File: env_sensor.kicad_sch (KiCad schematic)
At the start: 47 parts, among them J1 E Paper, J10 PWMOUT, J3 Barrel_Jack, J4 LED_OUTPUT, J5 RegSense, J6 I2c, J7 USB_C_Receptacle_USB2.0_16P, J8 v5_v3, J9 DEBUG, Q1 NMOS, Q2 NMOS, Q3 NMOS, SW1 EN, SW2 BOOT, U1 MH-Z19B, U3 ESP32-S3-WROOM-1, U4 TXB0104PW, U5 BME280, U6 TPS2065CDBV, U7 AP7361C-33E, Y1 Crystal

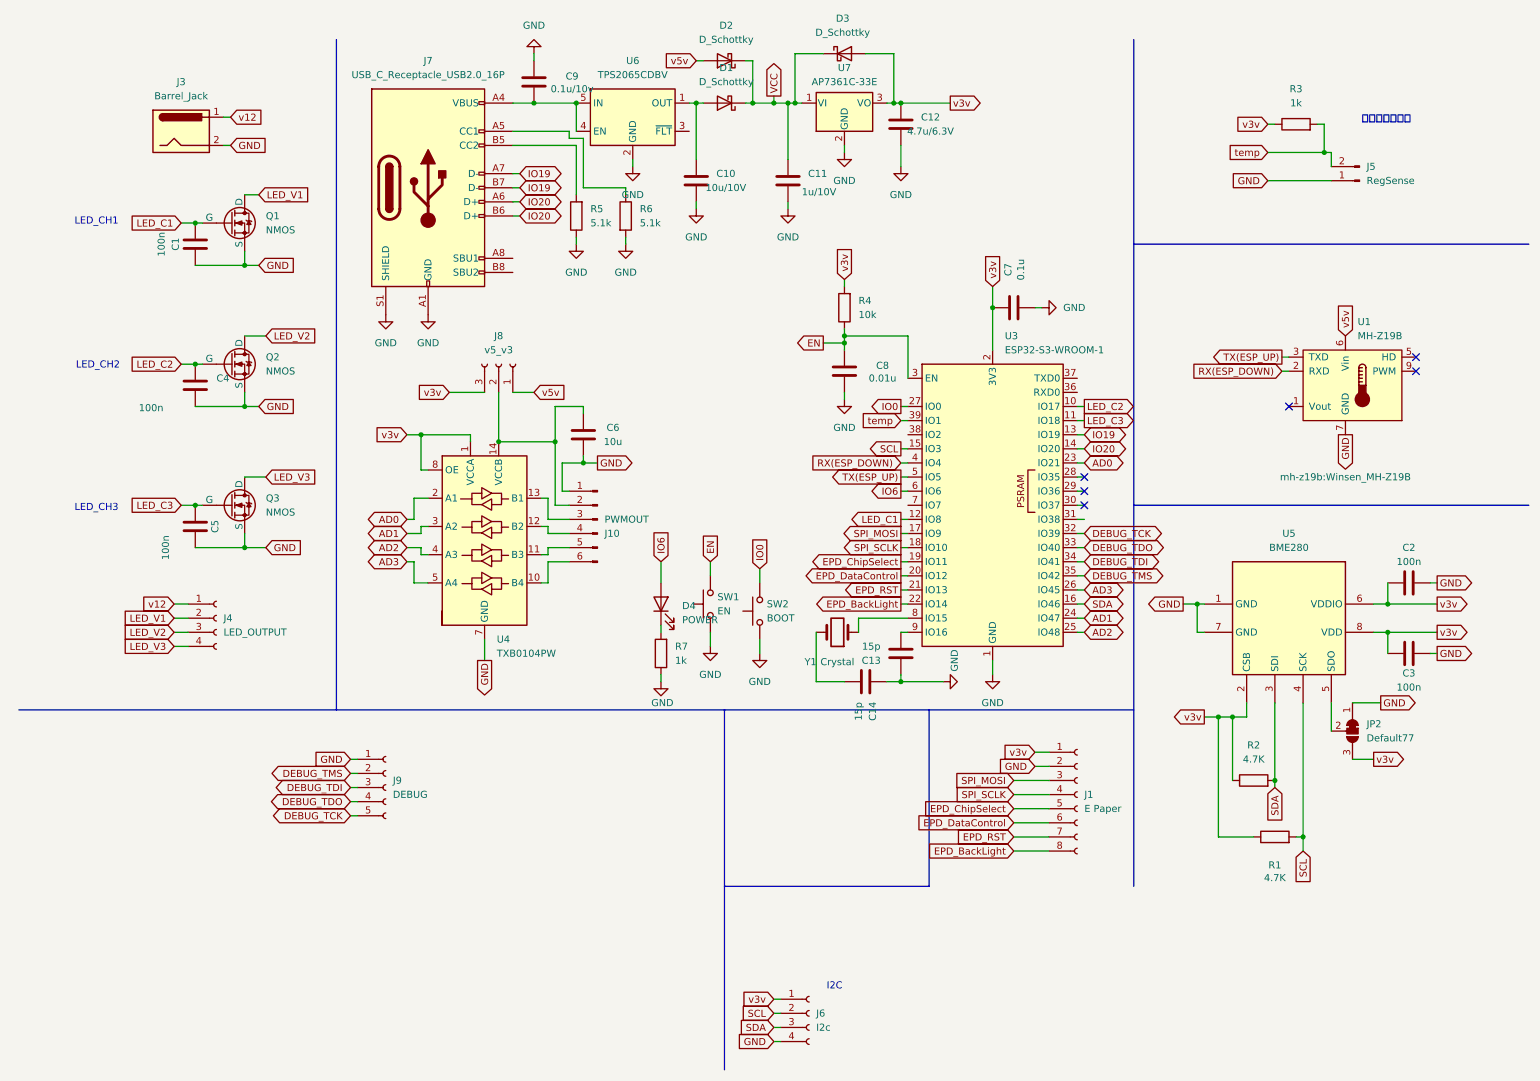
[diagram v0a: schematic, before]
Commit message: update
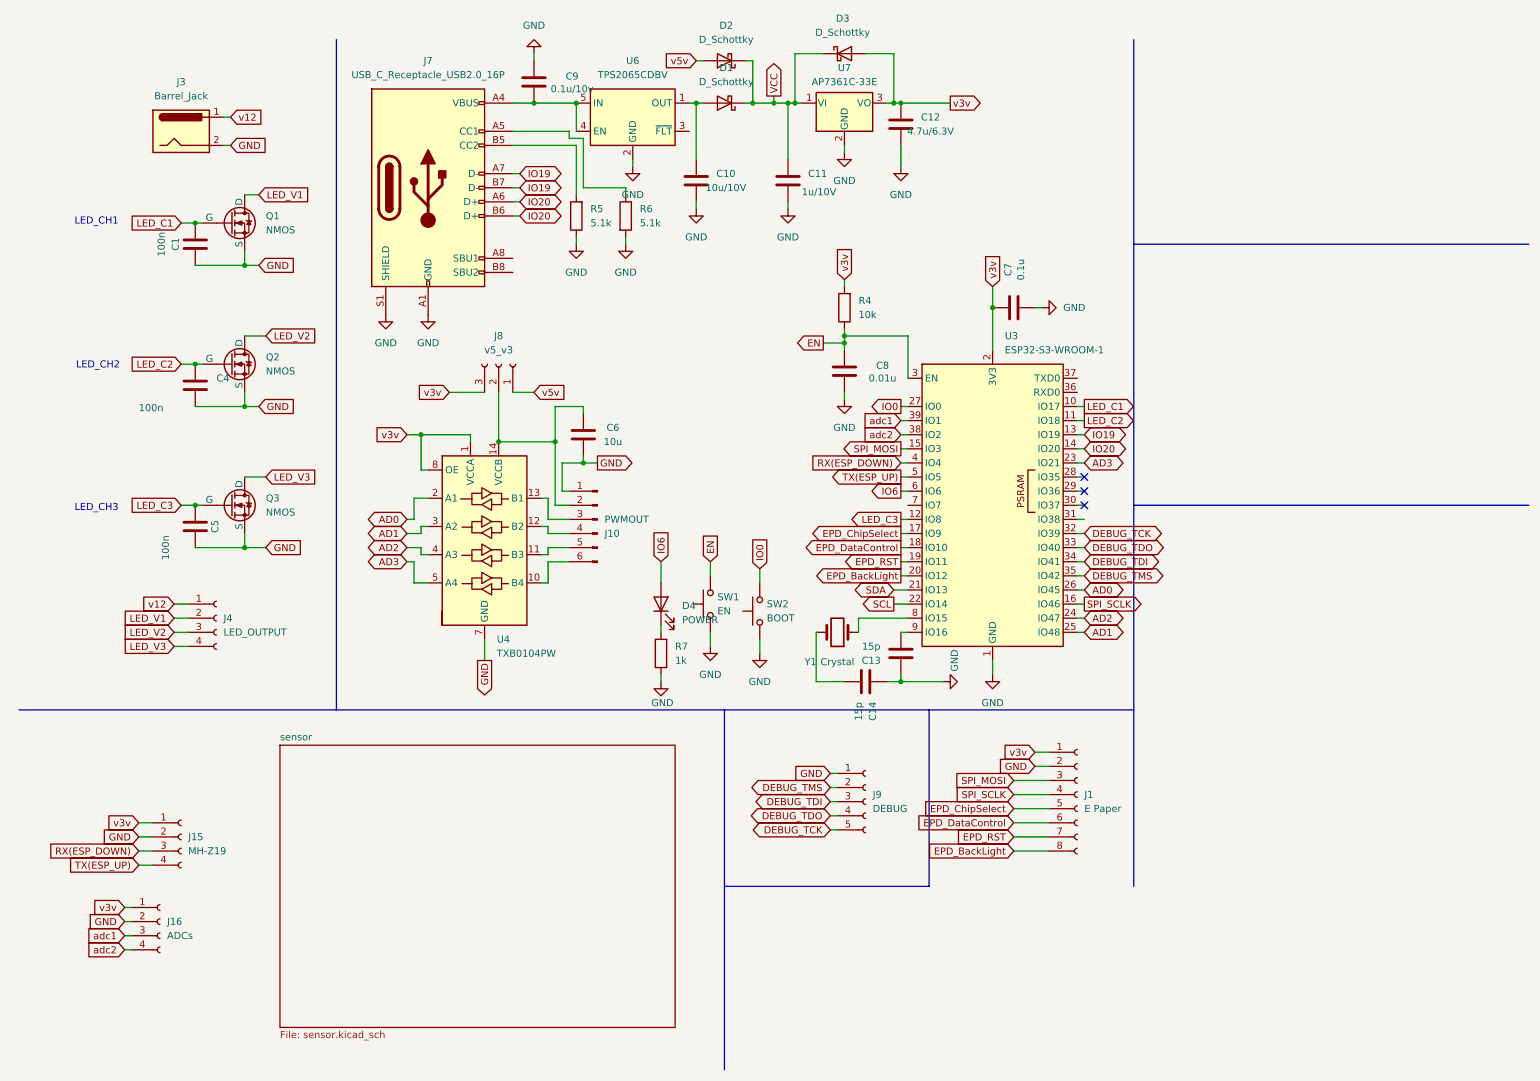
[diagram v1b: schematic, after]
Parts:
- removed C2, C3: 100n, Capacitor_SMD:C_0603_1608Metric, symbol Device:C
- removed J5: RegSense, Connector_PinSocket_2.54mm:PinSocket_1x02_P2.54mm_Vertical, symbol Connector:Conn_01x02_Pin
- removed J6: I2c, Connector_PinSocket_2.54mm:PinSocket_1x04_P2.54mm_Vertical, symbol Connector:Conn_01x04_Socket
- removed JP2: Default77, Jumper:SolderJumper-3_P1.3mm_Bridged12_RoundedPad1.0x1.5mm, symbol Jumper:SolderJumper_3_Bridged12
- removed R1, R2: 4.7K, Resistor_SMD:R_0603_1608Metric, symbol Device:R
- removed R3: 1k, Resistor_SMD:R_0603_1608Metric, symbol Device:R
- removed U1: MH-Z19B, mh-z19b:Winsen_MH-Z19B, symbol mh_z19b:MH-Z19B
- removed U5: BME280, Package_LGA:Bosch_LGA-8_2.5x2.5mm_P0.65mm_ClockwisePinNumbering, symbol Sensor:BME280
- added J15: MH-Z19, Connector_PinSocket_2.54mm:PinSocket_1x04_P2.54mm_Vertical, symbol Connector:Conn_01x04_Socket
- added J16: ADCs, Connector_PinSocket_2.54mm:PinSocket_1x04_P2.54mm_Vertical, symbol Connector:Conn_01x04_Socket
- Q1, Q2: footprint env-sensor:SOT-23 -> env-sensor:TO-252
- Q3: footprint env-sensor:SOT-23 -> env-sensor:TO-252; LCSC C916396 -> C557932
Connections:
- net AD0: now also U3.26 (IO45); no longer U3.23 (IO21)
- net AD1: now also U3.25 (IO48); no longer U3.24 (IO47)
- net AD2: now also U3.24 (IO47); no longer U3.25 (IO48)
- net AD3: now also U3.23 (IO21); no longer U3.26 (IO45)
- net EPD_BackLight: now also U3.20 (IO12); no longer U3.22 (IO14)
- net EPD_ChipSelect: now also U3.17 (IO9); no longer U3.19 (IO11)
- net EPD_DataControl: now also U3.18 (IO10); no longer U3.20 (IO12)
- net EPD_RST: now also U3.19 (IO11); no longer U3.21 (IO13)
- net GND: now also J15.2 (Pin_2), J16.2 (Pin_2)
- net LED_C1: now also U3.10 (IO17); no longer U3.12 (IO8)
- net LED_C2: now also U3.11 (IO18); no longer U3.10 (IO17)
- net LED_C3: now also U3.12 (IO8); no longer U3.11 (IO18)
- net RX(ESP_DOWN): now also J15.3 (Pin_3)
- net SCL: now also U3.22 (IO14); no longer U3.15 (IO3)
- net SDA: now also U3.21 (IO13); no longer U3.16 (IO46)
- net SPI_MOSI: now also U3.15 (IO3); no longer U3.17 (IO9)
- net SPI_SCLK: now also U3.16 (IO46); no longer U3.18 (IO10)
- net TX(ESP_UP): now also J15.4 (Pin_4)
- net v3v: now also J15.1 (Pin_1), J16.1 (Pin_1)
- net adc2: now reaches U3.38 (IO2)
- net adc2: now also J16.4 (Pin_4)
- net temp renamed adc1
- net adc1: now also J16.3 (Pin_3)
- no-connect marks 6 -> 3
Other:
- added sheet sensor (sensor.kicad_sch)
- note removed: "I2C"
- note removed: "サーミスタ回路"
- moved on the sheet: J9

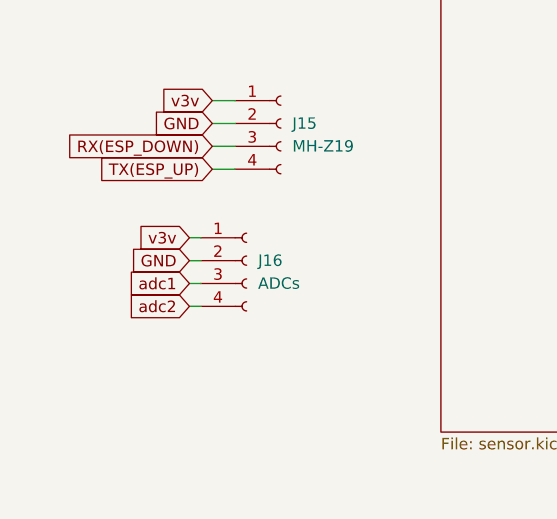
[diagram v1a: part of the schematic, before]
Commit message: fin
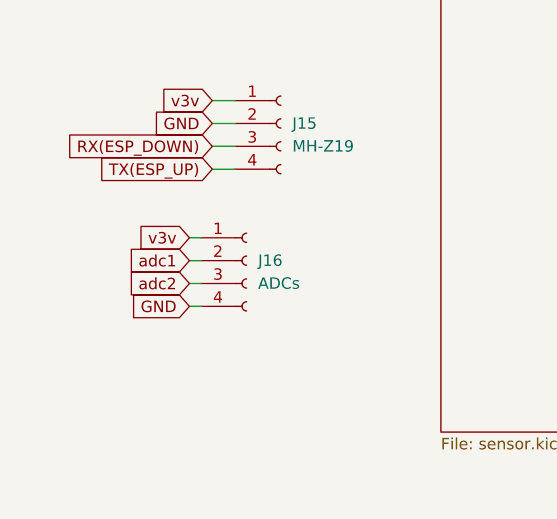
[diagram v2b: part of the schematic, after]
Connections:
- net GND: now also J16.4 (Pin_4); no longer J16.2 (Pin_2)
- net adc1: now also J16.2 (Pin_2); no longer J16.3 (Pin_3)
- net adc2: now also J16.3 (Pin_3); no longer J16.4 (Pin_4)
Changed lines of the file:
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@@
+		)
+	)
+	(global_label "adc2"
+		(shape input)
+		(at 31.75 173.99 180)
+		(fields_autoplaced yes)
+		(effects
+			(font
+				(size 1.27 1.27)
+			)
+			(justify right)
+		)
+		(property "Intersheetrefs" "${INTERSHEET_REFS}"
+			(at 24.1687 173.99 0)
+			(effects
+				(font
+					(size 1.27 1.27)
+				)
+				(justify right)
+				(hide yes)
+			)
 		)
 	)
@@
 		)
 	)
-	(global_label "adc1"
-		(shape input)
-		(at 31.75 173.99 180)
-		(fields_autoplaced yes)
-		(effects
-			(font
-				(size 1.27 1.27)
-			)
-			(justify right)
-		)
-		(property "Intersheetrefs" "${INTERSHEET_REFS}"
-			(at 24.1687 173.99 0)
-			(effects
-				(font
-					(size 1.27 1.27)
-				)
-				(justify right)
-				(hide yes)
-			)
-		)
-	)
 	(global_label "GND"
 		(shape input)
@@
 		)
 	)
-	(global_label "adc2"
-		(shape input)
-		(at 31.75 176.53 180)
-		(fields_autoplaced yes)
-		(effects
-			(font
-				(size 1.27 1.27)
-			)
-			(justify right)
-		)
-		(property "Intersheetrefs" "${INTERSHEET_REFS}"
-			(at 24.1687 176.53 0)
-			(effects
-				(font
-					(size 1.27 1.27)
-				)
-				(justify right)
-				(hide yes)
-			)
-		)
-	)
 	(global_label "LED_C1"
 		(shape input)
@@
 		)
 	)
+	(global_label "v5v"
+		(shape input)
+		(at 134.62 16.51 180)
+		(fields_autoplaced yes)
+		(effects
+			(font
+				(size 1.27 1.27)
+			)
+			(justify right)
+		)
+		(property "Intersheetrefs" "${INTERSHEET_REFS}"
+			(at 128.4901 16.51 0)
+			(effects
+				(font
+					(size 1.27 1.27)
+				)
+				(justify right)
+				(hide yes)
+			)
+		)
+	)
+	(global_label "adc1"
+		(shape input)
+		(at 31.75 171.45 180)
+		(fields_autoplaced yes)
+		(effects
+			(font
+				(size 1.27 1.27)
+			)
+			(justify right)
+		)
+		(property "Intersheetrefs" "${INTERSHEET_REFS}"
+			(at 24.1687 171.45 0)
+			(effects
+				(font
+					(size 1.27 1.27)
+				)
+				(justify right)
+				(hide yes)
+			)
+		)
+	)
+	(global_label "EPD_ChipSelect"
+		(shape input)
+		(at 191.77 151.13 180)
+		(fields_autoplaced yes)
+		(effects
+			(font
+				(size 1.27 1.27)
+			)
+			(justify right)
+		)
+		(property "Intersheetrefs" "${INTERSHEET_REFS}"
+			(at 174.0892 151.13 0)
+			(effects
+				(font
+					(size 1.27 1.27)
+				)
+				(justify right)
+				(hide yes)
+			)
+		)
+	)
 	(global_label "GND"
 		(shape input)
-		(at 31.75 171.45 180)
-		(fields_autoplaced yes)
-		(effects
-			(font
-				(size 1.27 1.27)
-			)
-			(justify right)
-		)
-		(property "Intersheetrefs" "${INTERSHEET_REFS}"
-			(at 24.8943 171.45 0)
-			(effects
-				(font
-					(size 1.27 1.27)
-				)
-				(justify right)
-				(hide yes)
-			)
-		)
-	)
-	(global_label "v5v"
-		(shape input)
-		(at 134.62 16.51 180)
-		(fields_autoplaced yes)
-		(effects
-			(font
-				(size 1.27 1.27)
-			)
-			(justify right)
-		)
-		(property "Intersheetrefs" "${INTERSHEET_REFS}"
-			(at 128.4901 16.51 0)
-			(effects
-				(font
-					(size 1.27 1.27)
-				)
-				(justify right)
-				(hide yes)
-			)
-		)
-	)
-	(global_label "EPD_ChipSelect"
-		(shape input)
-		(at 191.77 151.13 180)
-		(fields_autoplaced yes)
-		(effects
-			(font
-				(size 1.27 1.27)
-			)
-			(justify right)
-		)
-		(property "Intersheetrefs" "${INTERSHEET_REFS}"
-			(at 174.0892 151.13 0)
-			(effects
-				(font
+		(at 31.75 176.53 180)
+		(fields_autoplaced yes)
+		(effects
+			(font
+				(size 1.27 1.27)
+			)
+			(justify right)
+		)
+		(property "Intersheetrefs" "${INTERSHEET_REFS}"
+			(at 24.8943 176.53 0)
+			(effects
+				(font

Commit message: update lib for switch and fix DRCs
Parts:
- SW1, SW2: footprint (none) -> paripalpp_button:TVAF06-A020B-R
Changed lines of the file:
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@@
 			)
 		)
-		(property "Footprint" ""
+		(property "Footprint" "paripalpp_button:TVAF06-A020B-R"
 			(at 140.97 115.57 0)
 			(effects
@@
 			)
 		)
-		(property "Footprint" ""
+		(property "Footprint" "paripalpp_button:TVAF06-A020B-R"
 			(at 132.08 114.3 0)
 			(effects

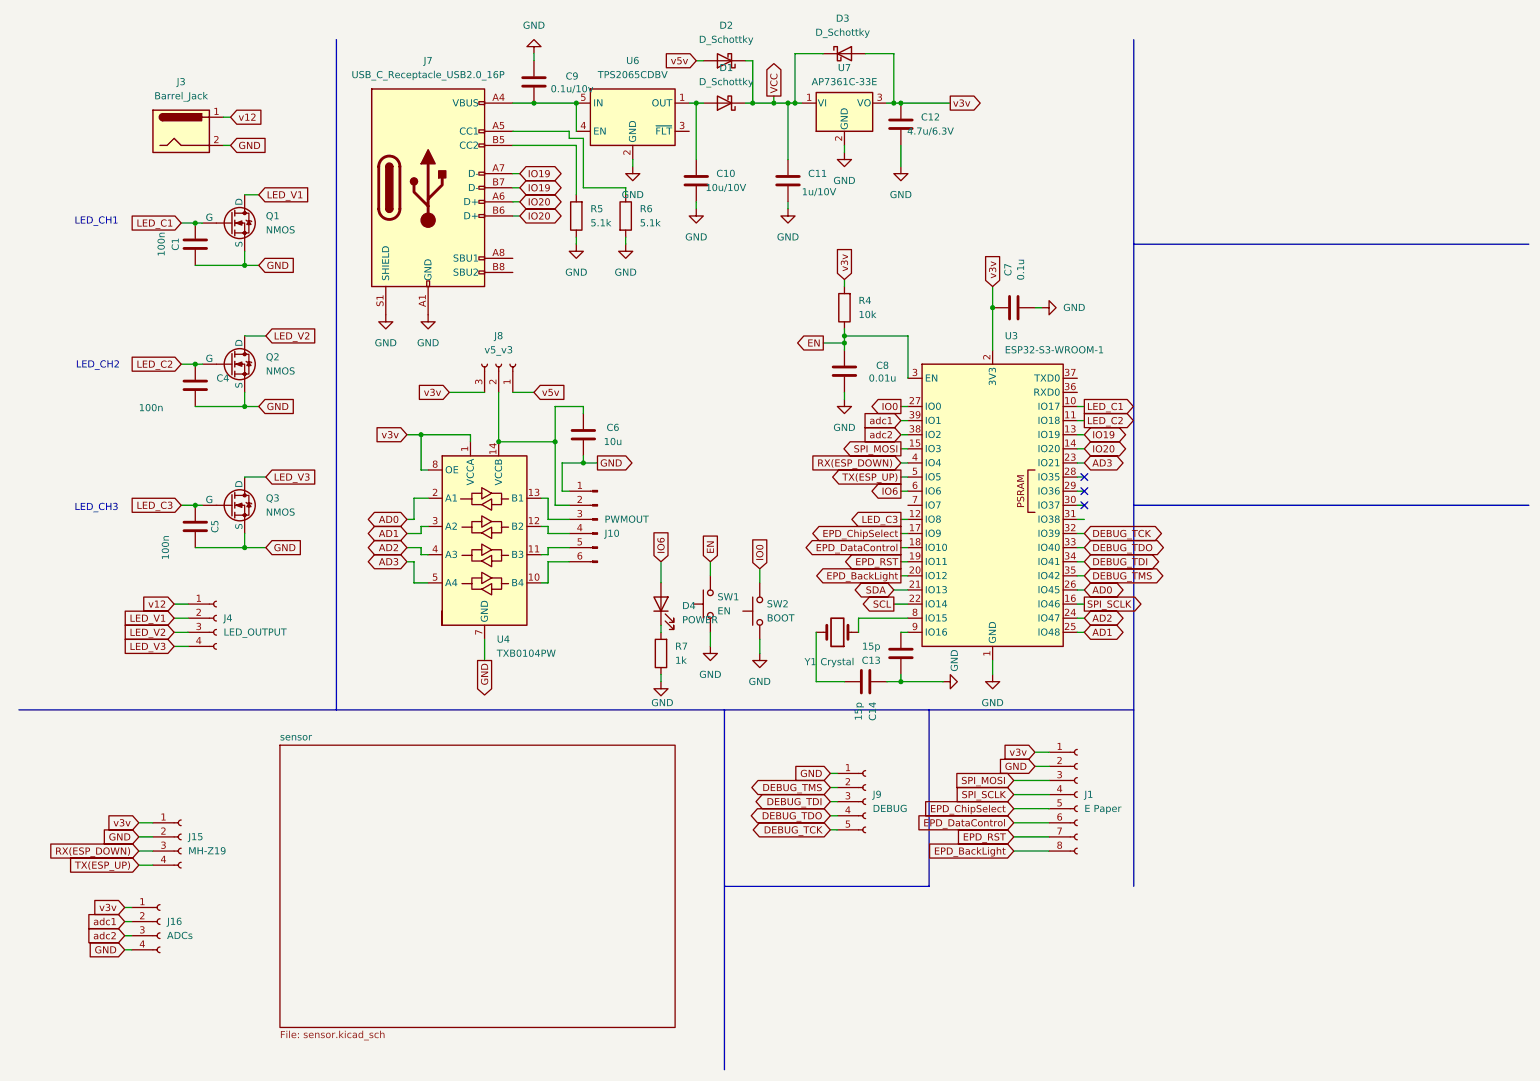
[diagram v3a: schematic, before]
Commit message: update
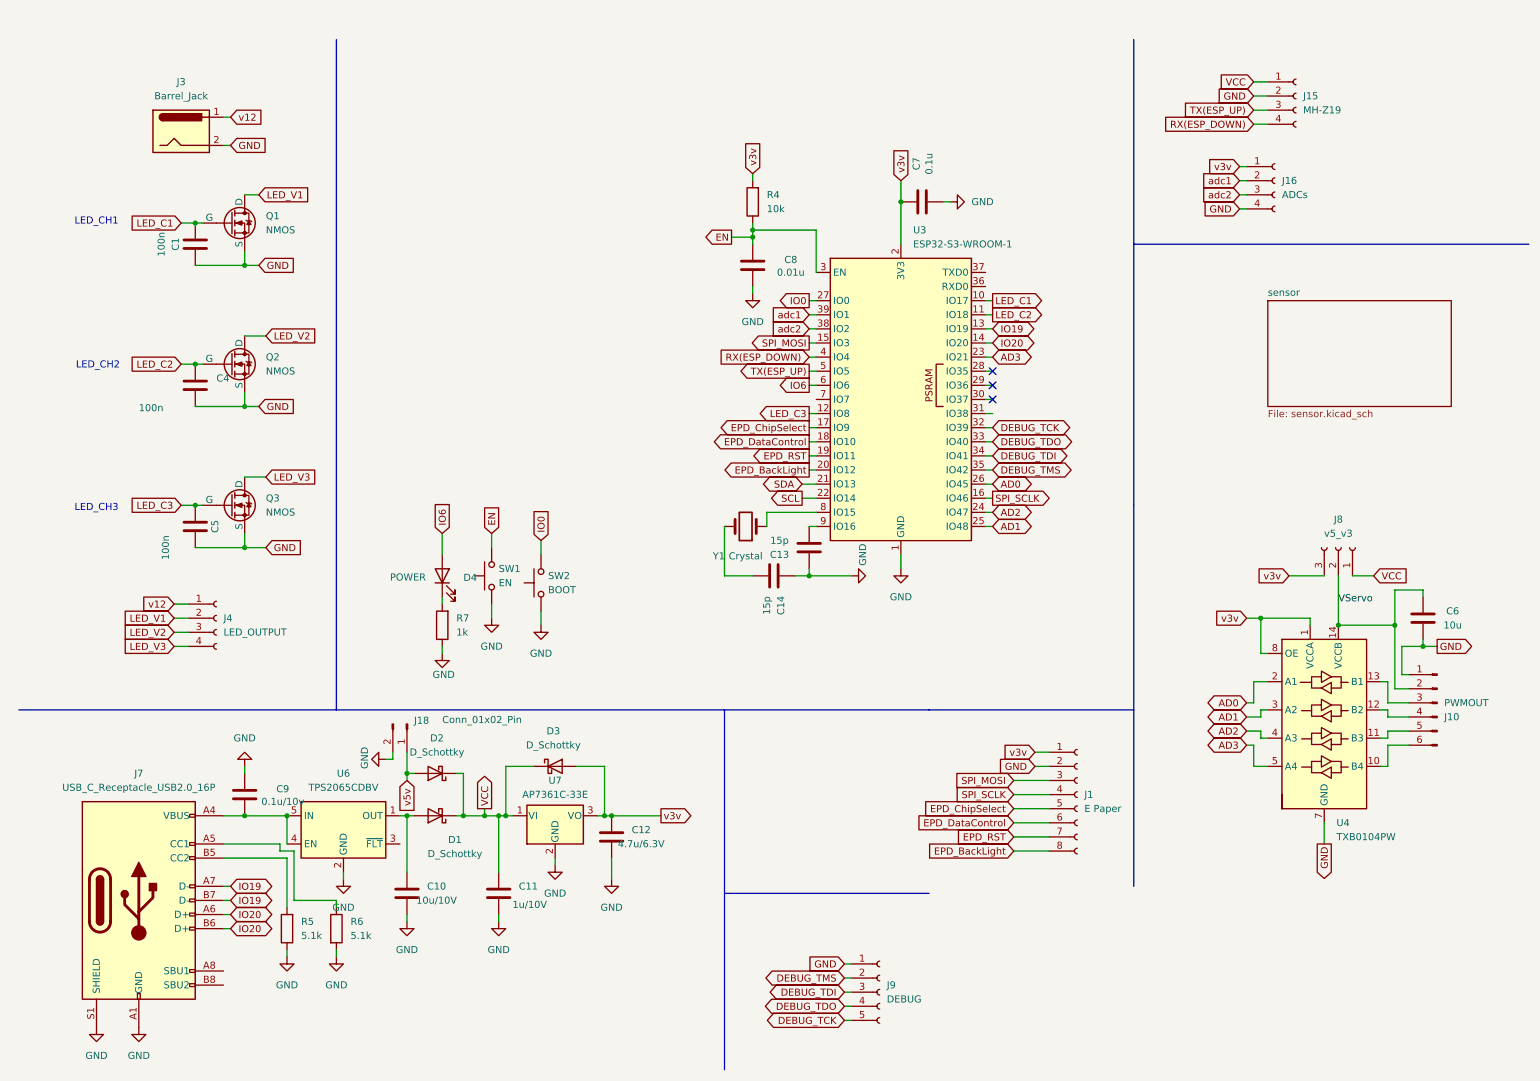
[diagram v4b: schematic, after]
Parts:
- added J18: Conn_01x02_Pin, Connector_PinHeader_2.54mm:PinHeader_1x02_P2.54mm_Vertical, symbol Connector:Conn_01x02_Pin
- J9: footprint Connector_PinSocket_2.54mm:PinSocket_1x05_P2.54mm_Vertical -> Connector_PinHeader_2.54mm:PinHeader_1x05_P2.54mm_Vertical
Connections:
- net GND: now also J18.2 (Pin_2)
- net RX(ESP_DOWN): now also J15.4 (Pin_4); no longer J15.3 (Pin_3)
- net TX(ESP_UP): now also J15.3 (Pin_3); no longer J15.4 (Pin_4)
- net VCC: now also J15.1 (Pin_1), J8.1 (Pin_1)
- net v3v: no longer J15.1 (Pin_1)
- net v5v: now also J18.1 (Pin_1); no longer J8.1 (Pin_1)
- net VServo: now reaches C6.1, J10.2 (Pin_2), J8.2 (Pin_2), U4.14 (VCCB)
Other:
- moved on the sheet: C10, C11, C12, C13, C14, C6, C7, C8, C9, D1, D2, D3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
